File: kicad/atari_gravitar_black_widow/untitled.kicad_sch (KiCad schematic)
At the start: 54 parts

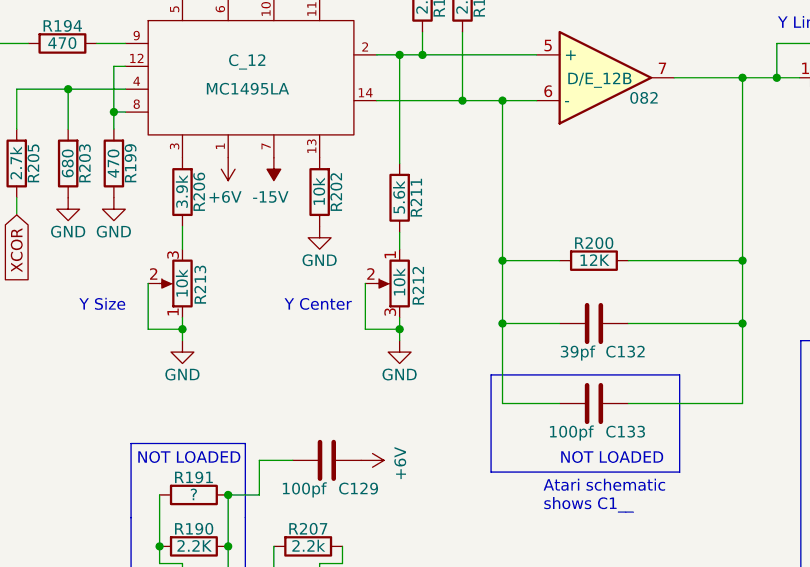
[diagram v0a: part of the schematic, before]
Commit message: Fixed various issues and generated gerber files
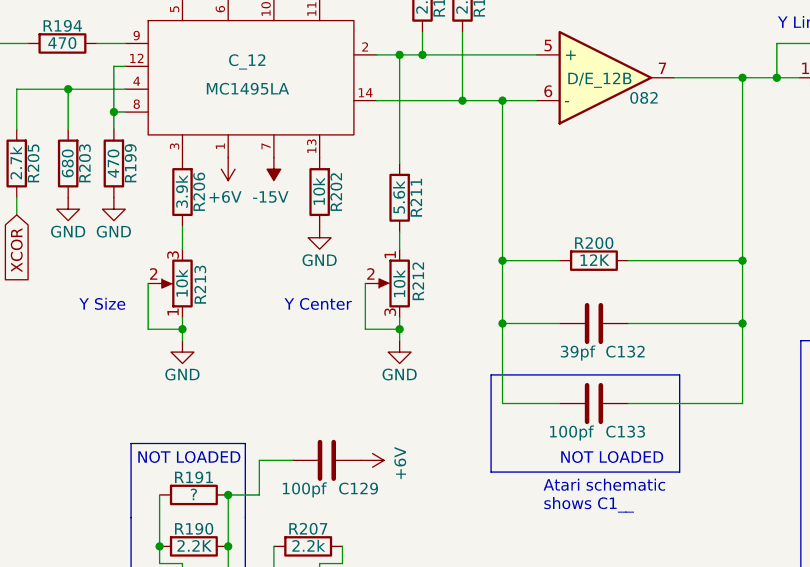
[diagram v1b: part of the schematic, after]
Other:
- moved on the sheet: R212
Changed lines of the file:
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@@
     (pin "1")
   )
-  (symbol (lib_name "POT_1") (lib_id "atari_grav_bw:POT") (at 478.536 192.786 180) (unit 1)
+  (symbol (lib_id "atari_grav_bw:POT") (at 478.536 192.786 0) (mirror y) (unit 1)
     (in_bom yes) (on_board yes)
-    (property "Reference" "R212" (id 0) (at 480.6607 195.3003 90)
+    (property "Reference" "R212" (id 0) (at 480.6607 190.2717 90)
       (effects (font (size 1.27 1.27)) (justify right))
     )
-    (property "Value" "10k" (id 1) (at 478.5714 194.3087 90)
+    (property "Value" "10k" (id 1) (at 478.5714 191.2633 90)
       (effects (font (size 1.27 1.27)) (justify right))
     )
